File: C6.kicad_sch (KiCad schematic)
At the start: 85 parts, among them J1 USB_C_Receptacle, J2 Battery_connector, J3 OLED-128x32, U1 rp2040-zero/xiao, U2 Seeeduino Xiao nRF52840

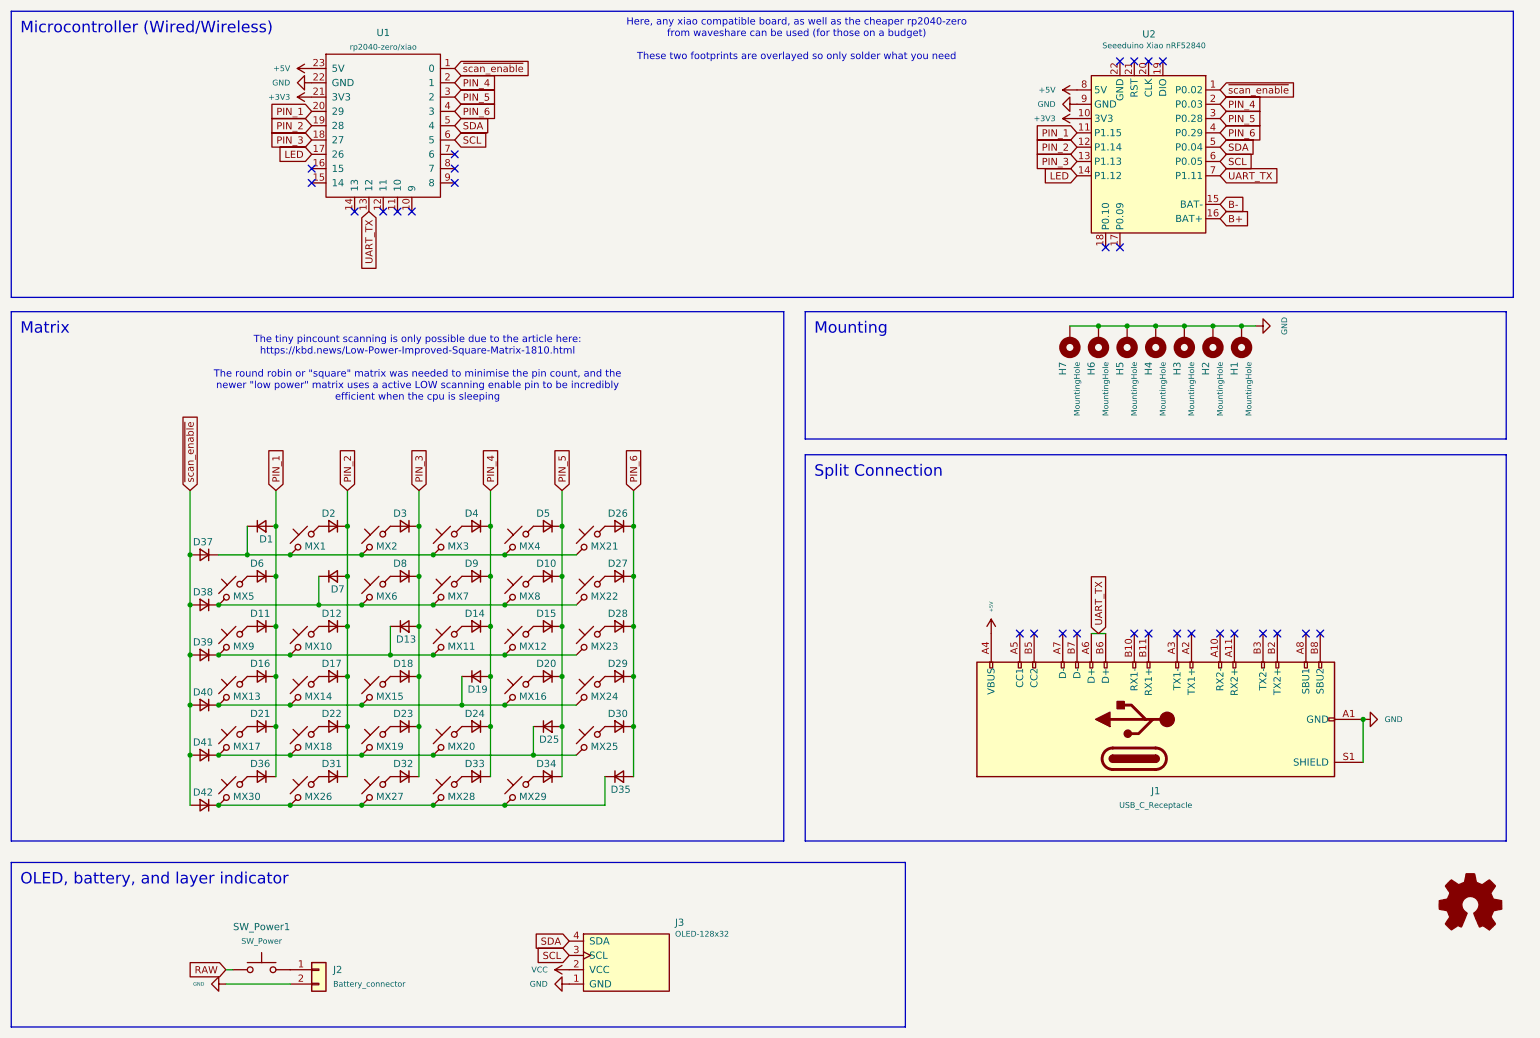
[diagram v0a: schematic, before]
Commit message: creation of PCB files
Signed-off-by: fami-fish <fami_fish@proton.me>
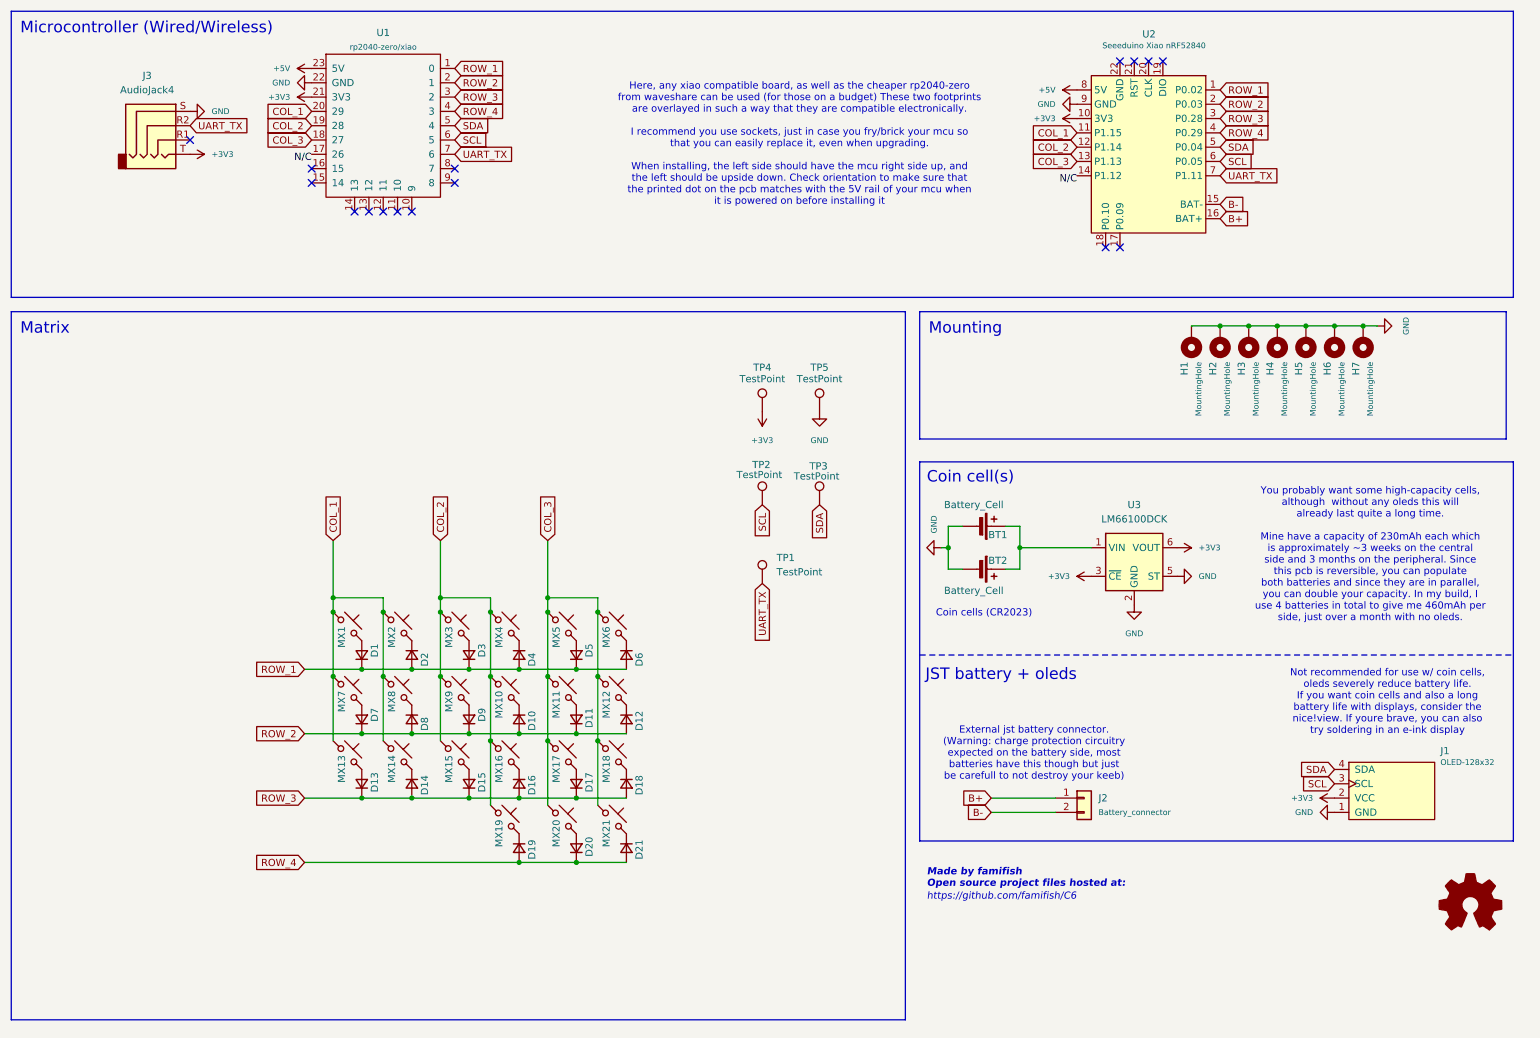
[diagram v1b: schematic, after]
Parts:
- removed D22, D23, D24, D25, D26, D27, D28, D29, D30, D31, D32, D33, D34, D35, D36, D37, D38, D39, D40, D41, D42: D_Small, Local:D_35, symbol Device:D_Small
- removed J1: USB_C_Receptacle, Connector_USB:USB_C_Receptacle_GCT_USB4085, symbol Connector:USB_C_Receptacle
- removed MX22, MX23, MX24, MX25, MX26, MX27, MX28, MX29, MX30: MX_SW_solder, Local:Reverisble_mx_choc_hybrid, symbol PCM_marbastlib-mx:MX_SW_solder
- removed SW_Power1: SW_Power, Button_Switch_THT:SW_DIP_SPSTx01_Slide_6.7x4.1mm_W7.62mm_P2.54mm_LowProfile, symbol Switch:SW_Push
- added BT1, BT2: Battery_Cell, misc:BatteryHolder_Keystone_3034_1x20mm_HandSolder_design, symbol Device:Battery_Cell
- added J3: AudioJack4, PCM_marbastlib-xp-various:CON_MJ-4PP-9_Reversible, symbol Connector_Audio:AudioJack4
- added TP1, TP2, TP3, TP4, TP5: TestPoint, TestPoint:TestPoint_Pad_D1.5mm, symbol Connector:TestPoint
- added U3: LM66100DCK, Package_TO_SOT_SMD:SOT-363_SC-70-6_Handsoldering, symbol Power_Management:LM66100DCK
- D1, D10, D11, D12, D13, D14, D15, D16, D17, D18, D19, D2, D20, D21, D3, D4, D5, D6, D7, D8, D9: footprint Local:D_35 -> misc:Diode_THT_SMD
- J2: footprint Connector_JST:JST_PH_B2B-PH-K_1x02_P2.00mm_Vertical -> misc:JST_PH_S2B-PH-K_1x02_P2.00mm_Horizontal_Reversible
- MX1, MX10, MX11, MX12, MX13, MX14, MX15, MX16, MX17, MX18, MX2, MX20, MX3, MX4, MX5, MX6, MX7, MX8, MX9: footprint Local:Reverisble_mx_choc_hybrid -> MX_V2_MX_Optional_Reversible:MX-Optional-Reversible-1U
- MX19, MX21: footprint Local:Reverisble_mx_choc_hybrid -> MX_V2_MX_Optional_Reversible:MX-Optional-Reversible-1.5U
- U1: footprint mcu:rp2040-zero-tht-pads -> mcu:rp2040-zero-tht
- renumbered H7 to H1, H6 to H2, H5 to H3, H3 to H5, H2 to H6, H1 to H7, J3 to J1
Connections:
- net VCC is gone; now on net +3V3: J1.2 (VCC)
- net +3V3: now also J3.T, TP4.1, U3.3 (~{CE}), U3.6 (VOUT)
- net B+: now also J2.1 (Pin_1)
- net B-: now also J2.2 (Pin_2)
- net GND: now also BT1.2 (-), BT2.2 (-), J3.S, TP5.1, U3.2 (GND), U3.5 (ST); no longer J2.2 (Pin_2)
- net SCL: now also TP2.1
- net SDA: now also TP3.1
- net UART_TX: now also U1.7 (6), J3.R2, TP1.1; no longer U1.13 (12)
- net at MX16.2: now also D16.1 (K); no longer D20.2 (A)
- net at MX14.2: now also D14.1 (K); no longer D17.2 (A)
- net at MX7.2: now also D7.2 (A); no longer D9.2 (A)
- net at MX5.2: now also D5.2 (A); no longer D6.2 (A)
- net at MX3.2: now also D3.2 (A); no longer D4.2 (A)
- net COL_3: now reaches MX17.1, MX18.1, MX20.1
- net COL_3: now also MX11.1, MX12.1, MX21.1, MX5.1, MX6.1, U1.18 (27), U2.13 (P1.13); no longer MX19.1
- net at MX17.2: now also D17.2 (A); no longer D21.2 (A)
- net at MX20.2: now also D20.2 (A)
- net at MX19.2: now also D19.1 (K)
- net at MX6.2: now also D6.1 (K); no longer D8.2 (A)
- net at MX18.2: now also D18.1 (K)
- net at MX11.2: now also D11.2 (A); no longer D14.2 (A)
- net at MX12.2: now also D12.1 (K); no longer D15.2 (A)
- net at MX21.2: now also D21.1 (K)
- net at MX2.2: now also D2.1 (K); no longer D3.2 (A)
- net at MX1.2: now also D1.2 (A); no longer D2.2 (A)
- net at MX15.2: now also D15.2 (A); no longer D18.2 (A)
- net at MX10.2: now also D10.1 (K); no longer D12.2 (A)
- net at MX9.2: now also D9.2 (A); no longer D11.2 (A)
- net at MX8.2: now also D8.1 (K); no longer D10.2 (A)
- net at MX13.2: now also D13.2 (A); no longer D16.2 (A)
- net at MX4.2: now also D4.1 (K); no longer D5.2 (A)
- net LED renamed N/C
- removed net PIN_1: D1.2 (A), D11.1 (K), D16.1 (K), D21.1 (K), D6.1 (K), U1.20 (29), U2.11 (P1.15)
- removed net PIN_2: D12.1 (K), D17.1 (K), D2.1 (K), D7.2 (A), U1.19 (28), U2.12 (P1.14)
- removed net PIN_3: D13.2 (A), D18.1 (K), D3.1 (K), D8.1 (K), U1.18 (27), U2.13 (P1.13)
- net PIN_4 renamed ROW_2
- net ROW_2: now also D10.2 (A), D11.1 (K), D12.2 (A), D7.1 (K), D8.2 (A); no longer D14.1 (K), D19.2 (A), D4.1 (K)
- net PIN_5 renamed ROW_3
- net ROW_3: now also D13.1 (K), D14.2 (A), D16.2 (A), D17.1 (K), D18.2 (A); no longer D10.1 (K), D20.1 (K), D5.1 (K)
- net PIN_6 renamed ROW_4
- net ROW_4: now also D19.2 (A), D20.1 (K), D21.2 (A)
- net ~{scan_enable} renamed ROW_1
- net ROW_1: now also D1.1 (K), D2.2 (A), D3.1 (K), D4.2 (A), D5.1 (K), D6.2 (A)
- new net: BT1.1 (+), BT2.1 (+), U3.1 (VIN)
- new net COL_1: MX1.1, MX13.1, MX14.1, MX2.1, MX7.1, MX8.1, U1.20 (29), U2.11 (P1.15)
- new net COL_2: MX10.1, MX15.1, MX16.1, MX19.1, MX3.1, MX4.1, MX9.1, U1.19 (28), U2.12 (P1.14)
- no-connect marks 29 -> 16
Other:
- note added: "Coin cell(s)"
- note added: "Coin cells (CR2023)"
- note added: "External jst battery connector. (Warning: charge protection circuitry expected on the battery side, most batteries have this though but just be carefull to not destroy your keeb)"
- note added: "Here, any xiao compatible board, as well as the cheaper rp2040-zero from waveshare can be used (for those on a budget) These two footprints are overlayed in such a way that they are compatible electronically. I recommend you use sockets, just in case you fry/brick your mcu so that you can easily replace it, even when upgrading. When installing, the left side should have the mcu right side up, and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"
- note added: "JST battery + oleds"
- note added: "Made by famifish Open source project files hosted at:"
- note added: "Not recommended for use w/ coin cells, oleds severely reduce battery life. If you want coin cells and also a long battery life with displays, consider the nice!view. If youre brave, you can also try soldering in an e-ink display"
- note added: "You probably want some high-capacity cells, although without any oleds this will already last quite a long time. Mine have a capacity of 230mAh each which is approximately ~3 weeks on the central side and 3 months on the peripheral. Since this pcb is reversible, you can populate both batteries and since they are in parallel, you can double your capacity. In my build, I use 4 batteries in total to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"
- note added: "https://github.com/famifish/C6"
- note removed: "Here, any xiao compatible board, as well as the cheaper rp2040-zero from waveshare can be used (for those on a budget) These two footprints are overlayed so only solder what you need"
- note removed: "The tiny pincount scanning is only possible due to the article here: https://kbd.news/Low-Power-Improved-Square-Matrix-1810.html The round robin or "square" matrix was needed to minimise the pin count, and the newer "low power" matrix uses a active LOW scanning enable pin to be incredibly efficient when the cpu is sleeping"
- title: (none) -> C6
- moved on the sheet: H1, H2, H3, H4, H5, H6, H7, J1, J2
